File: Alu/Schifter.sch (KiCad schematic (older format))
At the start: 0 parts

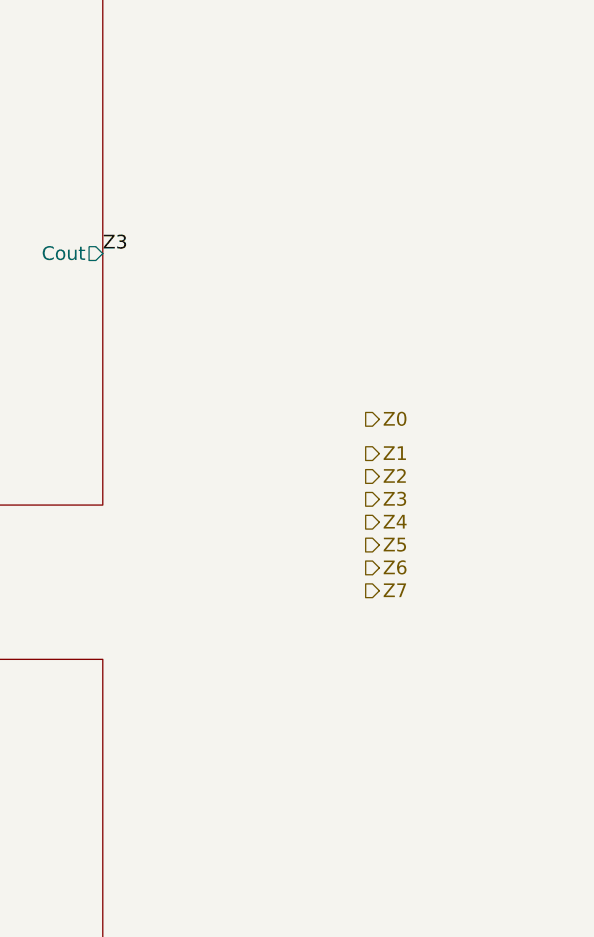
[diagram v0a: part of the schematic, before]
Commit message: footprints
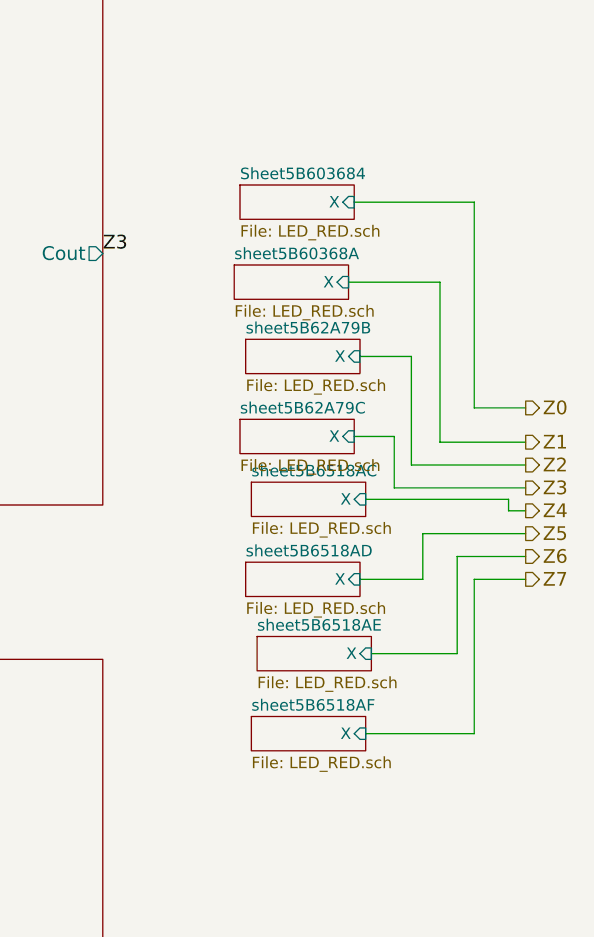
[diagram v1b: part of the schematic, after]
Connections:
- wire segments 377 -> 401
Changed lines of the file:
@@
 $Descr A3 16535 11693
 encoding utf-8
-Sheet 107 156
+Sheet 116 191
 Title ""
 Date ""
@@
 Text Label 13500 6050 0    60   ~ 0
 Z7
-Text HLabel 14650 3400 2    60   Output ~ 0
+Text HLabel 15350 3350 2    60   Output ~ 0
 Z0
-Text HLabel 14650 3550 2    60   Output ~ 0
+Text HLabel 15350 3500 2    60   Output ~ 0
 Z1
-Text HLabel 14650 3650 2    60   Output ~ 0
+Text HLabel 15350 3600 2    60   Output ~ 0
 Z2
-Text HLabel 14650 3750 2    60   Output ~ 0
+Text HLabel 15350 3700 2    60   Output ~ 0
 Z3
-Text HLabel 14650 3850 2    60   Output ~ 0
+Text HLabel 15350 3800 2    60   Output ~ 0
 Z4
-Text HLabel 14650 3950 2    60   Output ~ 0
+Text HLabel 15350 3900 2    60   Output ~ 0
 Z5
-Text HLabel 14650 4050 2    60   Output ~ 0
+Text HLabel 15350 4000 2    60   Output ~ 0
 Z6
-Text HLabel 14650 4150 2    60   Output ~ 0
+Text HLabel 15350 4100 2    60   Output ~ 0
 Z7
 Text Label 2175 6475 2    50   ~ 0
@@
 Wire Wire Line
 	2175 3425 2175 3475
+$Sheet
+S 14100 2375 500  150
+U 5B603685
+F0 "Sheet5B603684" 50
+F1 "LED_RED.sch" 50
+F2 "X" I R 14600 2450 50
+$EndSheet
+$Sheet
+S 14075 2725 500  150
+U 5B60368D
+F0 "sheet5B60368A" 50
+F1 "LED_RED.sch" 50
+F2 "X" I R 14575 2800 50
+$EndSheet
+$Sheet
+S 14125 3050 500  150
+U 5B62A79F
+F0 "sheet5B62A79B" 50
+F1 "LED_RED.sch" 50
+F2 "X" I R 14625 3125 50
+$EndSheet
+$Sheet
+S 14100 3400 500  150
+U 5B62A7A2
+F0 "sheet5B62A79C" 50
+F1 "LED_RED.sch" 50
+F2 "X" I R 14600 3475 50
+$EndSheet
+$Sheet
+S 14150 3675 500  150
+U 5B6518B2
+F0 "sheet5B6518AC" 50
+F1 "LED_RED.sch" 50
+F2 "X" I R 14650 3750 50
+$EndSheet
+$Sheet
+S 14125 4025 500  150
+U 5B6518B5
+F0 "sheet5B6518AD" 50
+F1 "LED_RED.sch" 50
+F2 "X" I R 14625 4100 50
+$EndSheet
+$Sheet
+S 14175 4350 500  150
+U 5B6518B8
+F0 "sheet5B6518AE" 50
+F1 "LED_RED.sch" 50
+F2 "X" I R 14675 4425 50
+$EndSheet
+$Sheet
+S 14150 4700 500  150
+U 5B6518BB
+F0 "sheet5B6518AF" 50
+F1 "LED_RED.sch" 50
+F2 "X" I R 14650 4775 50
+$EndSheet
+Wire Wire Line
+	14600 2450 15125 2450
+Wire Wire Line
+	15125 2450 15125 3350
+Wire Wire Line
+	15125 3350 15350 3350
+Wire Wire Line
+	15350 3500 14975 3500
+Wire Wire Line
+	14975 3500 14975 2800
+Wire Wire Line
+	14975 2800 14575 2800
+Wire Wire Line
+	14625 3125 14850 3125
+Wire Wire Line
+	14850 3125 14850 3600
+Wire Wire Line
+	14850 3600 15350 3600
+Wire Wire Line
+	14600 3475 14775 3475
+Wire Wire Line
+	14775 3475 14775 3700
+Wire Wire Line
+	14775 3700 15350 3700
+Wire Wire Line
+	14650 3750 15275 3750
+Wire Wire Line
+	15275 3750 15275 3800
+Wire Wire Line
+	15275 3800 15350 3800
+Wire Wire Line
+	15350 3900 14900 3900
+Wire Wire Line
+	14900 3900 14900 4100
+Wire Wire Line
+	14900 4100 14625 4100
+Wire Wire Line
+	14675 4425 15050 4425
+Wire Wire Line
+	15050 4425 15050 4000
+Wire Wire Line
+	15050 4000 15350 4000
+Wire Wire Line
+	15350 4100 15125 4100
+Wire Wire Line
+	15125 4100 15125 4775
+Wire Wire Line
+	15125 4775 14650 4775
 $EndSCHEMATC
